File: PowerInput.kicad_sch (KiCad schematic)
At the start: 16 parts, among them J17 V_{IN}, Q1 Q_PMOS_GSD, Q2 Q_PMOS_GSD

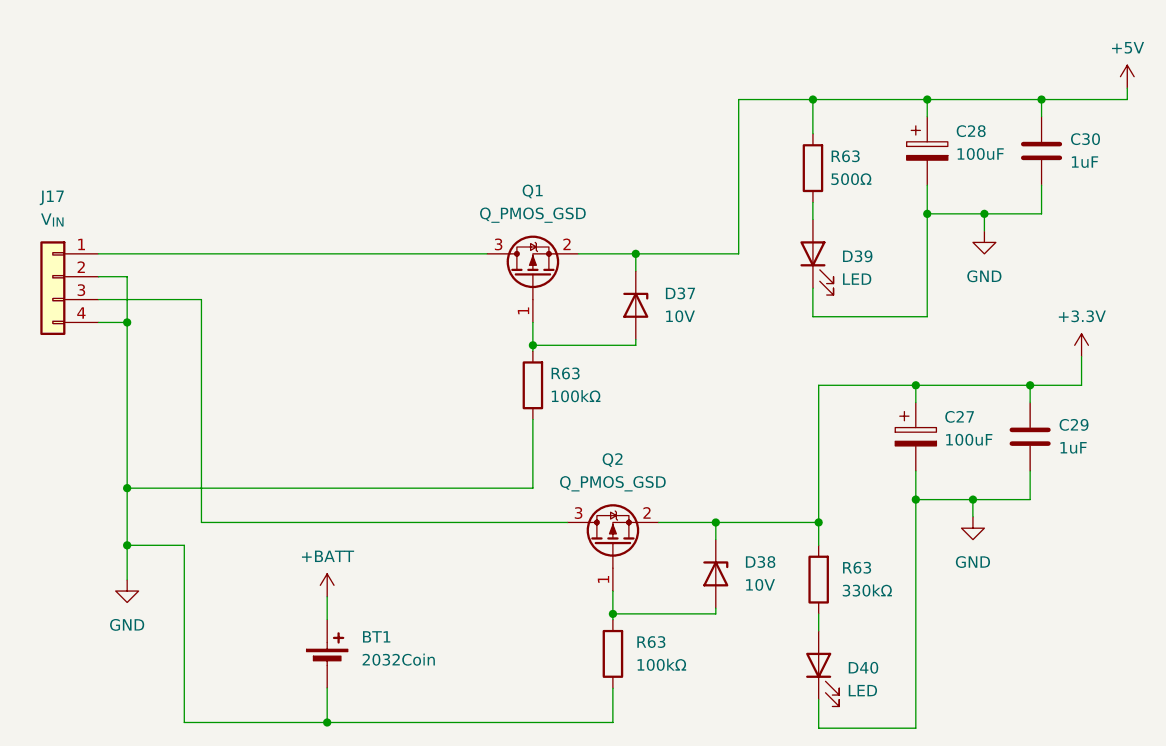
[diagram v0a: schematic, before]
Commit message: Initial commit.
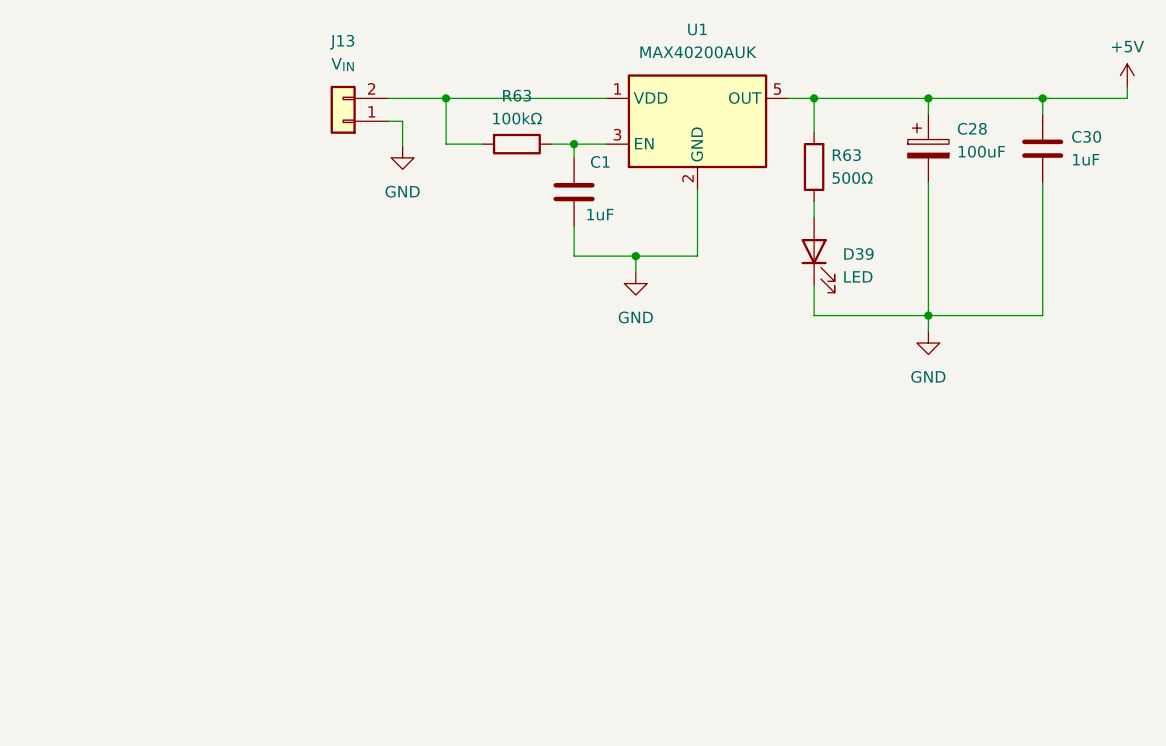
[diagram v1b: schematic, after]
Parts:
- removed BT1: 2032Coin, BatteryCoin:BC2032, symbol Device:Battery_Cell
- removed C27: 100uF, Capacitor_SMD:CP_Elec_8x11.9, symbol Device:C_Polarized
- removed C29: 1uF, Capacitor_SMD:C_0805_2012Metric, symbol Device:C
- removed D37, D38: 10V, Diode_SMD:D_SOD-123, symbol Device:D_Zener
- removed D40: LED, LED_SMD:LED_0805_2012Metric, symbol Device:LED
- removed J17: V_{IN}, TerminalBlock:TerminalBlock_bornier-4_P5.08mm, symbol Connector_Generic:Conn_01x04
- removed Q1, Q2: Q_PMOS_GSD, Package_TO_SOT_SMD:SOT-23, symbol Device:Q_PMOS_GSD
- removed R63 (x2): 100kΩ, Resistor_SMD:R_0805_2012Metric, symbol Device:R
- removed R63: 330kΩ, Resistor_SMD:R_0805_2012Metric, symbol Device:R
- added C1: 1uF, Capacitor_SMD:C_0805_2012Metric, symbol Device:C
- added J13: V_{IN}, Connector_PinHeader_2.54mm:PinHeader_1x02_P2.54mm_Vertical, symbol Connector_Generic:Conn_01x02
- added R63: 100kΩ, Resistor_SMD:R_0805_2012Metric, symbol Device:R
- added U1: MAX40200AUK, Package_TO_SOT_SMD:SOT-23-5, symbol Analog_Switch:MAX40200AUK
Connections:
- net +5V: now also U1.5 (OUT)
- net GND: now also C1.2, J13.1 (Pin_1), U1.2 (GND)
- new net: J13.2 (Pin_2), R63.2, U1.1 (VDD)
- new net: C1.1, R63.1, U1.3 (EN)
